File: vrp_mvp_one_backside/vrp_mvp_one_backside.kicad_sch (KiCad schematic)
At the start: 12 parts, among them J1 USB_C_Receptacle_USB2.0_16P, J2 BACKSIDE_INTERFACE, J7 BACKSIDE_INTERFACE_2, Q2 MMBT2222A

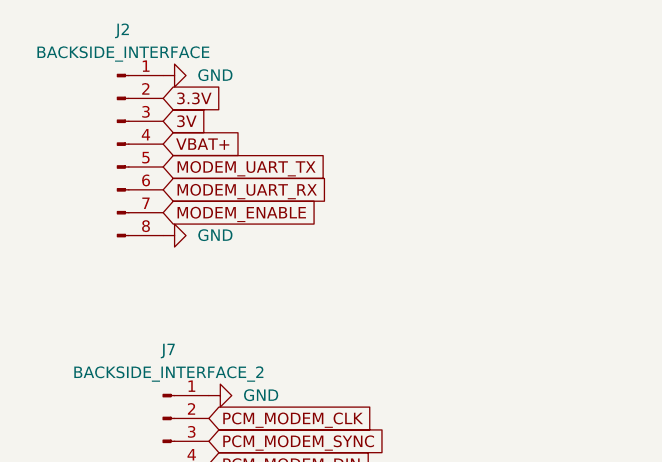
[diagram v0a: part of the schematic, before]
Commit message: more routing and part placement
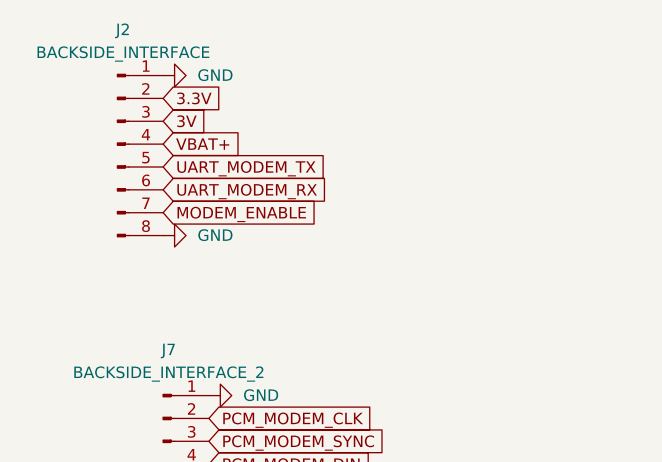
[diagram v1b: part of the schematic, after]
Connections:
- net MODEM_UART_RX renamed UART_MODEM_RX
- net MODEM_UART_TX renamed UART_MODEM_TX
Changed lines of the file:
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@@
 		)
 	)
-	(global_label "MODEM_UART_TX"
+	(global_label "UART_MODEM_TX"
 		(shape input)
 		(at 36.83 38.1 0)
@@
 		)
 	)
-	(global_label "MODEM_UART_RX"
+	(global_label "UART_MODEM_RX"
 		(shape input)
 		(at 36.83 40.64 0)

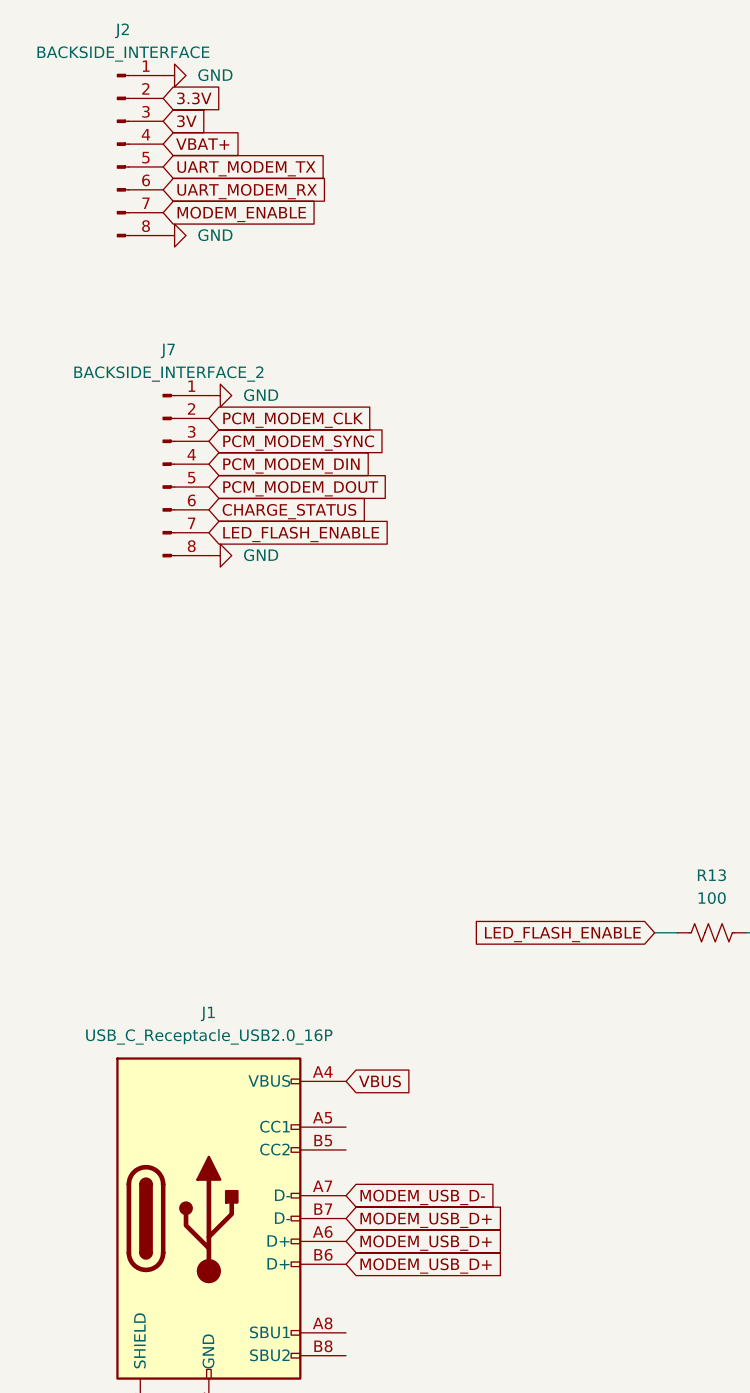
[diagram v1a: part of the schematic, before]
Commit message: changes
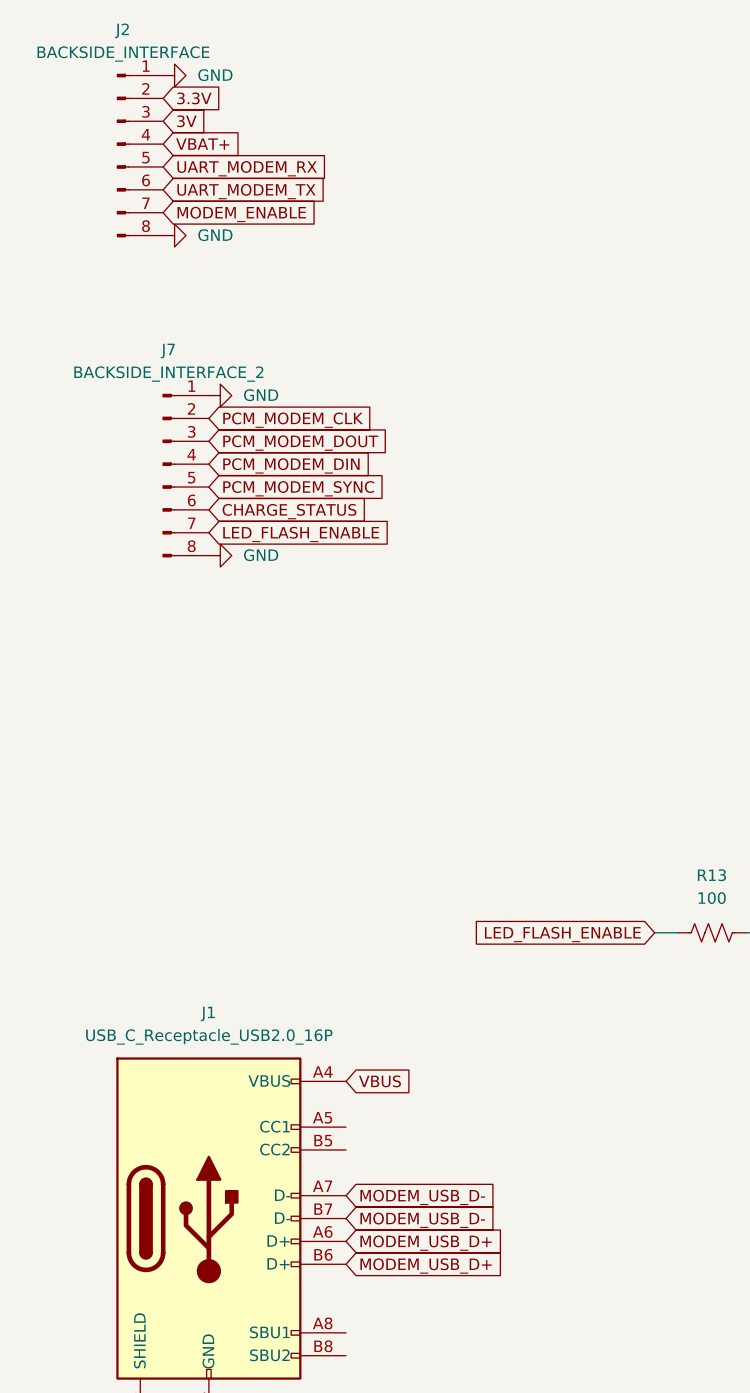
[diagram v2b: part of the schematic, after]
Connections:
- net MODEM_USB_D+: no longer J1.B7 (D-)
- net MODEM_USB_D-: now also J1.B7 (D-)
- net PCM_MODEM_DOUT: now also J7.3 (Pin_3); no longer J7.5 (Pin_5)
- net PCM_MODEM_SYNC: now also J7.5 (Pin_5); no longer J7.3 (Pin_3)
- net UART_MODEM_RX: now also J2.5 (Pin_5); no longer J2.6 (Pin_6)
- net UART_MODEM_TX: now also J2.6 (Pin_6); no longer J2.5 (Pin_5)
